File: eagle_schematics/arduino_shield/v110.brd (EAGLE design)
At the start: 100 x 80 mm, 10 parts, among them U1 ARDUINO_SHIELDLABEL

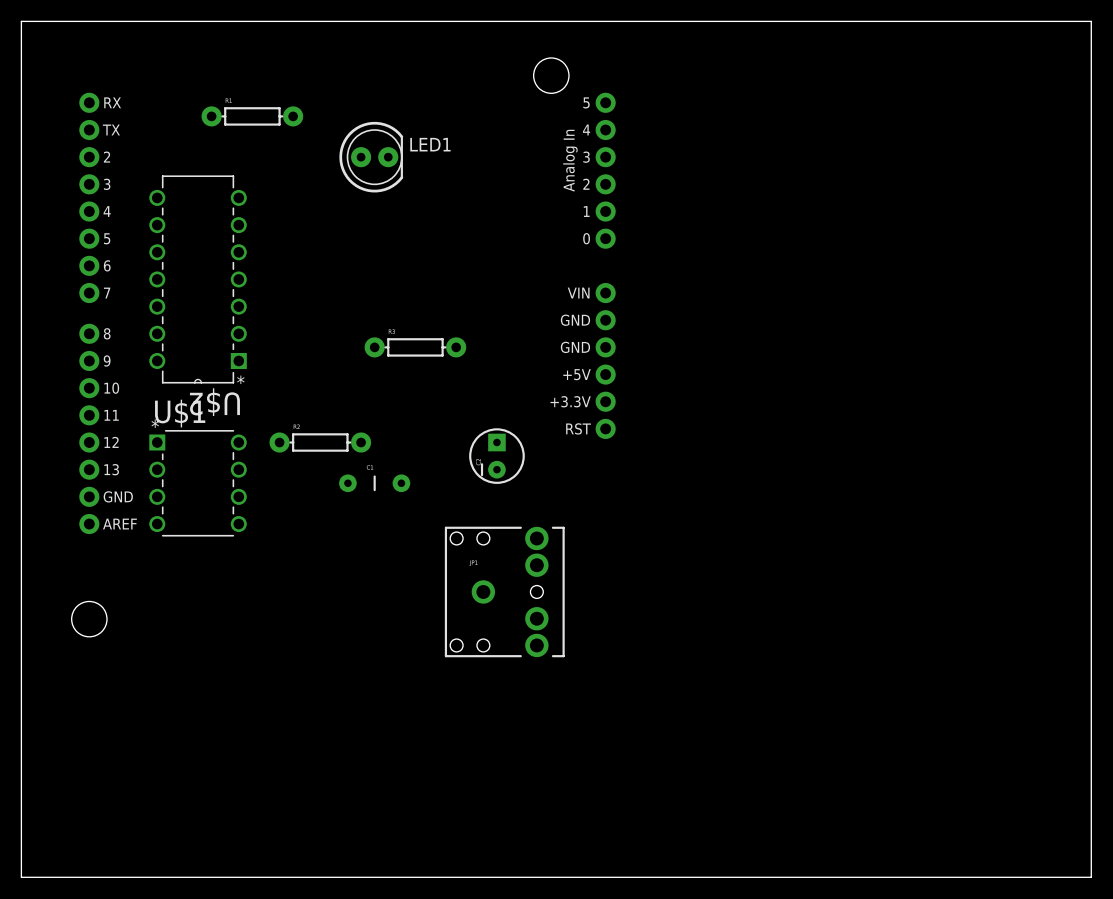
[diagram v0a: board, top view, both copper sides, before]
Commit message: new board rev
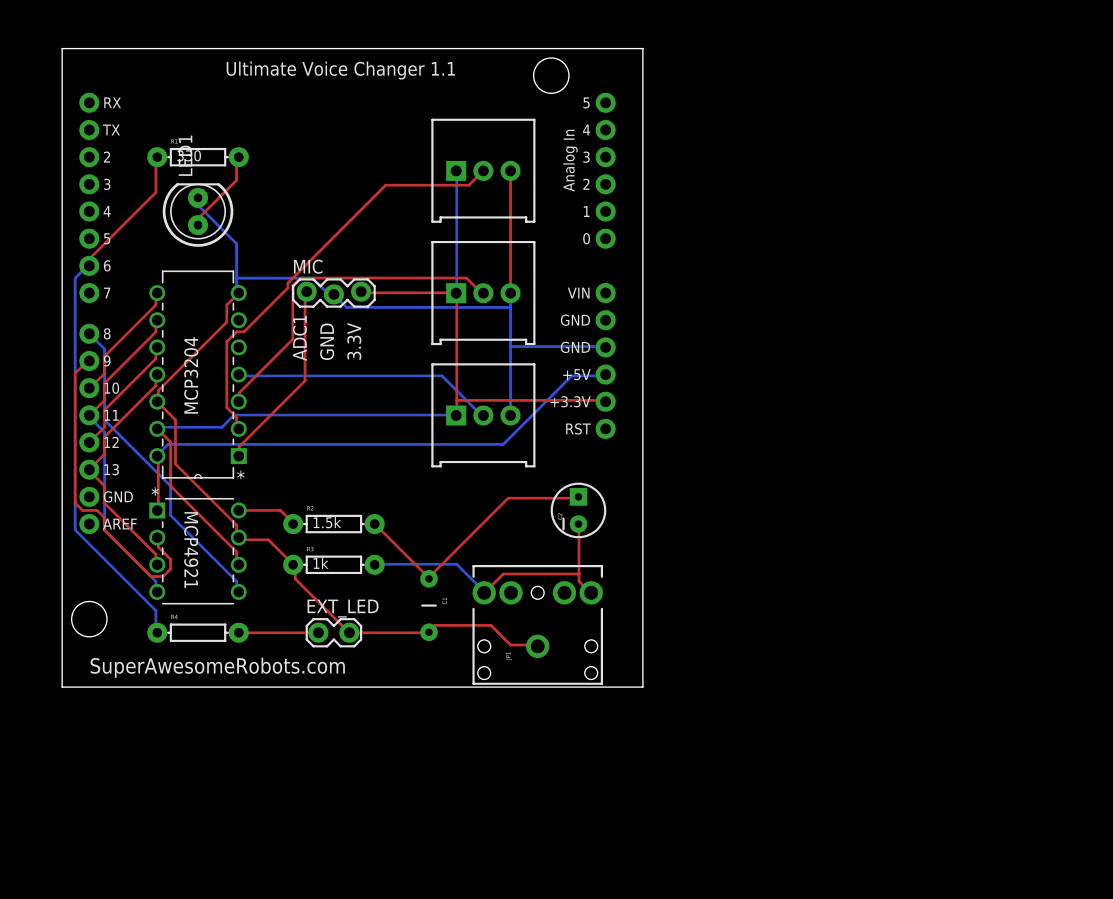
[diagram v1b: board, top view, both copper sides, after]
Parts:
- added ADC2, ADC3, ADC4: TRIMPOT-PTH-KNOB, SparkFun-Electromechanical:3386U
- added EXT_LED: M02LOCK, SparkFun-Connectors:1X02_LOCK
- added MIC: (no value), SparkFun-Connectors:1X03_LOCK
- added R4: (no value), SparkFun-Resistors:AXIAL-0.3
- C1: value (none) -> 0.1uF
- C2: value (none) -> 10uF
- R1: value (none) -> 330
- R2: value (none) -> 1.5k
- R3: value (none) -> 1k
- moved R3 21.7 mm to (29.2, 29.2)
- moved LED1 17.3 mm to (16.5, 62.2), turned to 90 degrees
- moved C1 12.5 mm to (38.1, 25.4), turned to 270 degrees
- moved C2 9.16 mm to (52.1, 34.3)
- moved U$2 8.89 mm to (12.7, 54.6)
- moved R2 7.73 mm to (29.2, 33.0)
- moved JP1 7.18 mm to (48.3, 21.6), turned to 90 degrees
- moved U$1 6.35 mm to (20.3, 26.7)
- moved R1 6.35 mm to (16.5, 67.3)
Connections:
- new net N$5: EXT_LED.1, R4.P$2
- net 3.3V: now also ADC2.1, ADC3.1, ADC4.1, MIC.3
- net ADC1: now also MIC.1
- net ADC2: now also ADC2.2
- net ADC3: now also ADC3.2
- net ADC4: now also ADC4.2
- net GND: now also ADC2.3, ADC3.3, ADC4.3, EXT_LED.2, MIC.2
- net LED: now also R4.P$1, U1.D6
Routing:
- net GND: track 0.00 -> 131.9 mm
- net 3.3V: track 0.00 -> 90.3 mm
- net LED: track 0.00 -> 51.0 mm
- net 5V: track 0.00 -> 50.3 mm
- net ADC2: track 0.00 -> 39.5 mm
- net ADC3: track 0.00 -> 31.6 mm
- net MOSI: track 0.00 -> 30.7 mm
- net CS_DAC: track 0.00 -> 30.1 mm
- net LDAC: track 0.00 -> 30.0 mm
- net N$4: track 0.00 -> 27.9 mm
- net ADC4: track 0.00 -> 24.5 mm
- net N$3: track 0.00 -> 24.4 mm
- net SCK: track 0.00 -> 23.1 mm
- net ADC1: track 0.00 -> 18.0 mm
- net CS_ADC: track 0.00 -> 11.5 mm
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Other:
- board size 100 x 80 mm -> 54.3 x 59.7 mm
- board text added: "3.3V"
- board text added: "ADC1"
- board text added: "GND"
- board text added: "MCP3204"
- board text added: "MCP4921"
- board text added: "SuperAwesomeRobots.com"
- board text added: "Ultimate Voice Changer 1.1"
